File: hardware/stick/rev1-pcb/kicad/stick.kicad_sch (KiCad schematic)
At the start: 0 parts

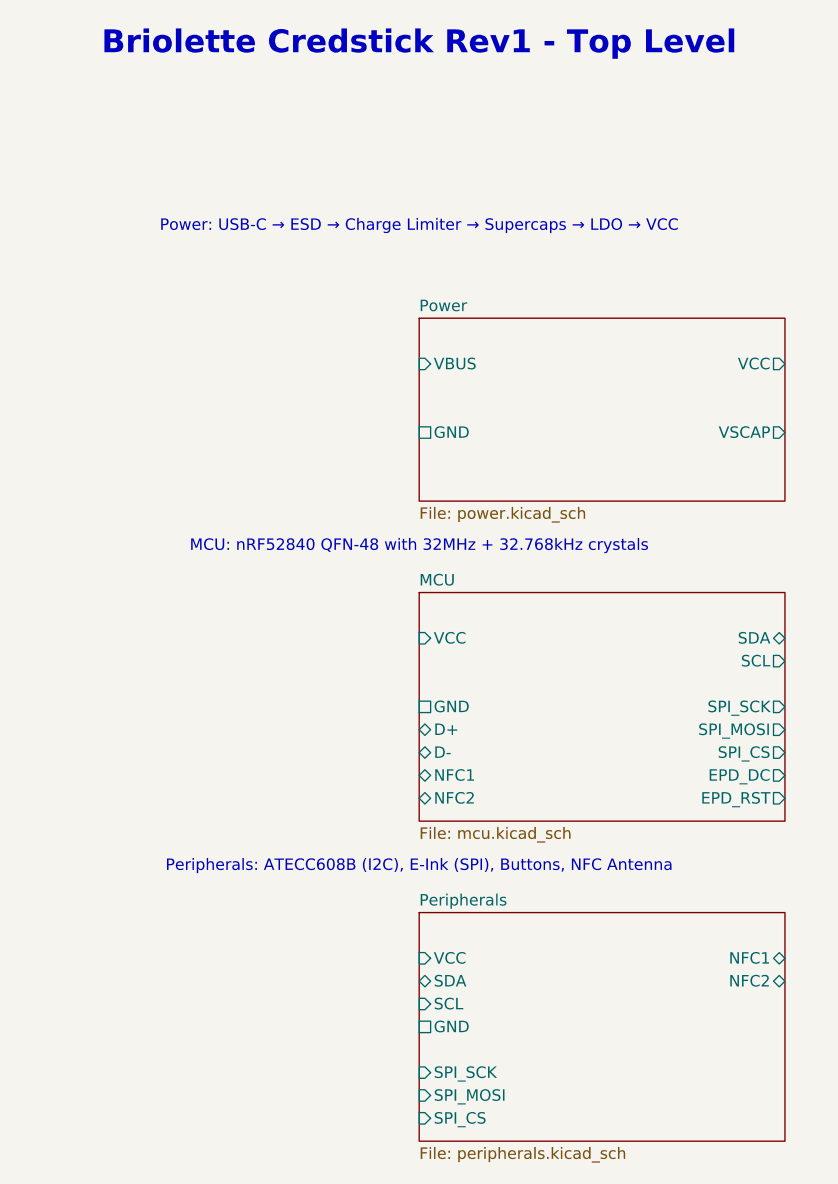
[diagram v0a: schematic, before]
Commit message: Replace ATECC608B with nano-SIM in push-push connector, add concurrent init
Replace the soldered-down ATECC608B secure element with a user-replaceable
nano-SIM card in a low-profile push-push connector (Molex 78800-0001,
1.25mm height). The SIM provides the same tamper-resistant functions
(P-256 ECDSA, key storage, monotonic counters) via standard ISO 7816
interface, but is field-swappable for identity transfer or replacement.
This makes the prototype robust enough for production use.

Hardware changes:
- Peripherals schematic: ATECC608B U5 → J3 nano-SIM connector
- I2C (SDA/SCL) → ISO 7816 (SIM_IO, SIM_CLK, SIM_RST, SIM_DET)
- MCU GPIO reassignment: P0.26=SIM_IO, P0.27=SIM_CLK, P0.22=SIM_RST,
  P0.24=SIM_DET
- New KiCad symbol (NanoSIM_PushPush) and footprint (NanoSIM_Molex_78800)
- BOM updated: SIM connector + card replaces ATECC608B
- 3D case: added SIM card slot cutout in side wall

Firmware changes:
- New sim_card.rs: async ISO 7816 T=0 driver over UARTE, with ATR
  parsing, applet selection, INTERNAL AUTHENTICATE signing, GET DATA
  for certificates/keys, and monotonic counter operations
- main.rs: concurrent initialization using embassy_futures::join3 —
  storage init, SIM card init, and display setup run in parallel
- Switched from blocking I2C (twim) to async UARTE for SIM communication
- atecc608b.rs marked deprecated (retained for reference)

https://claude.ai/code/session_01TM1rFxbipYtvAkh4Vt7My7
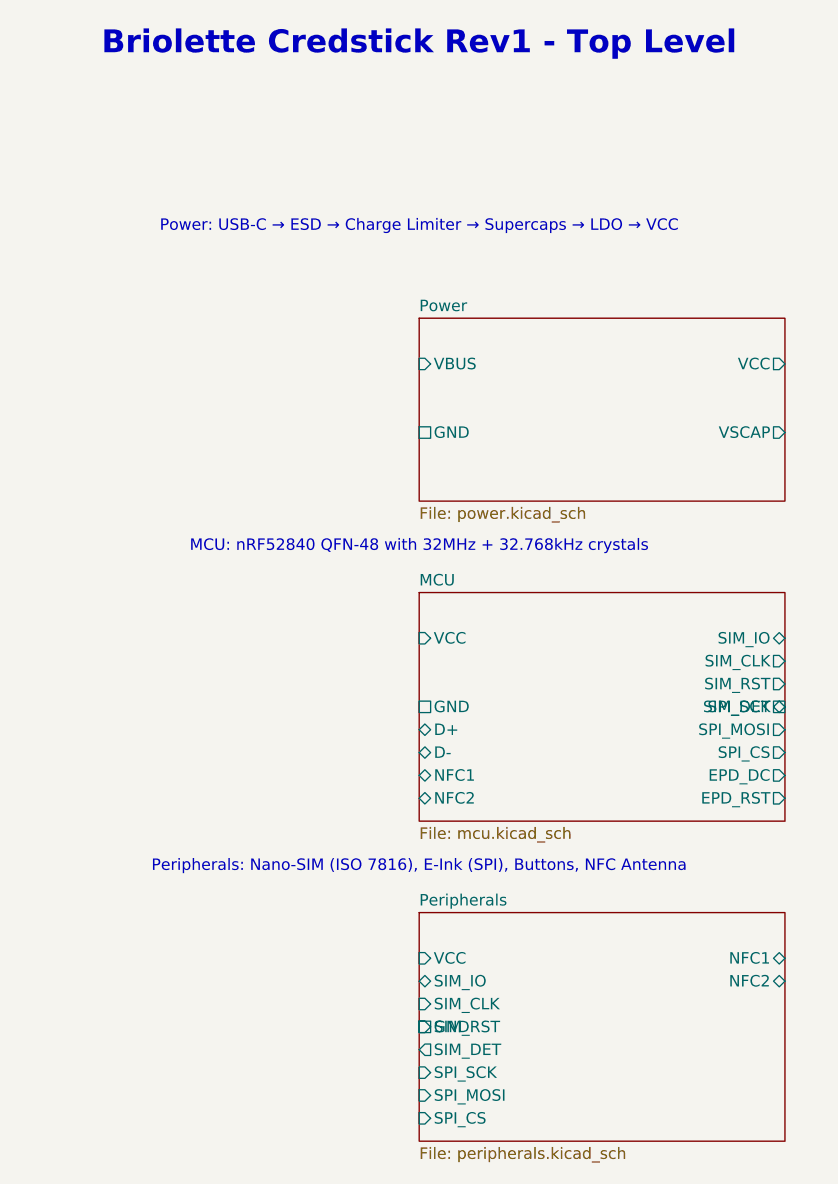
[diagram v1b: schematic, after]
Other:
- sheet MCU ports: added SIM_CLK, SIM_DET, SIM_IO, SIM_RST; removed SCL, SDA
- sheet Peripherals ports: added SIM_CLK, SIM_DET, SIM_IO, SIM_RST; removed SCL, SDA
- note added: "Peripherals: Nano-SIM (ISO 7816), E-Ink (SPI), Buttons, NFC Antenna"
- note removed: "Peripherals: ATECC608B (I2C), E-Ink (SPI), Buttons, NFC Antenna"
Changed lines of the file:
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@@
     (rev "1.0")
     (comment 1 "4-layer PCB, 60x30mm keychain form factor")
-    (comment 2 "nRF52840 + ATECC608B + E-Ink + NFC")
+    (comment 2 "nRF52840 + Nano-SIM (ISO 7816) + E-Ink + NFC")
   )
   ;; ============================================================
@@
       (effects (font (size 1.27 1.27)) (justify left))
     )
-    (pin "SDA" bidirectional
+    (pin "SIM_IO" bidirectional
       (at 66.04 86.36 0)
       (effects (font (size 1.27 1.27)) (justify right))
     )
-    (pin "SCL" output
+    (pin "SIM_CLK" output
       (at 66.04 88.9 0)
+      (effects (font (size 1.27 1.27)) (justify right))
+    )
+    (pin "SIM_RST" output
+      (at 66.04 91.44 0)
+      (effects (font (size 1.27 1.27)) (justify right))
+    )
+    (pin "SIM_DET" input
+      (at 66.04 93.98 0)
       (effects (font (size 1.27 1.27)) (justify right))
     )
@@
   )
   ;; ============================================================
-  ;; Sheet: Peripherals (ATECC608B, E-Ink, Buttons, NFC antenna)
+  ;; Sheet: Peripherals (Nano-SIM, E-Ink, Buttons, NFC antenna)
   ;; ============================================================
   (sheet
@@
       (effects (font (size 1.27 1.27)) (justify left))
     )
-    (pin "SDA" bidirectional
+    (pin "SIM_IO" bidirectional
       (at 25.4 124.46 180)
       (effects (font (size 1.27 1.27)) (justify left))
     )
-    (pin "SCL" input
+    (pin "SIM_CLK" input
       (at 25.4 127 180)
+      (effects (font (size 1.27 1.27)) (justify left))
+    )
+    (pin "SIM_RST" input
+      (at 25.4 129.54 180)
+      (effects (font (size 1.27 1.27)) (justify left))
+    )
+    (pin "SIM_DET" output
+      (at 25.4 132.08 180)
       (effects (font (size 1.27 1.27)) (justify left))
     )
@@
     (effects (font (size 1.27 1.27)))
   )
-  (text "Peripherals: ATECC608B (I2C), E-Ink (SPI), Buttons, NFC Antenna"
+  (text "Peripherals: Nano-SIM (ISO 7816), E-Ink (SPI), Buttons, NFC Antenna"
     (exclude_from_sim no)
     (at 25.4 111.76 0)
